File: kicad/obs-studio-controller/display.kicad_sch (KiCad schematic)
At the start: 3 parts, among them J4 Conn_Display, Q1 2N7002

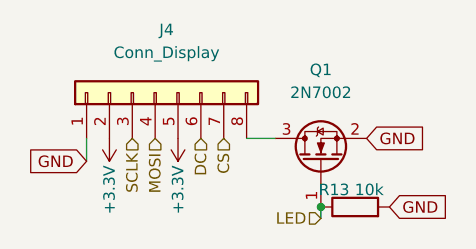
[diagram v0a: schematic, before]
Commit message: Routing complete
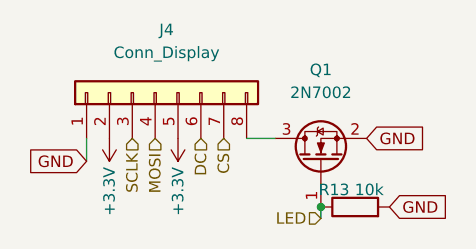
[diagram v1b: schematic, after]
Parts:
- J4: footprint Connector_PinHeader_2.54mm:PinHeader_1x08_P2.54mm_Vertical -> custom:DISPLAY
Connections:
- net +3.3V renamed +3V3
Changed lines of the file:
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@@
     (effects (font (size 1.27 1.27)) (justify right))
+  )
+  (symbol (lib_id "power:+3.3V") (at 34.925 30.48 180) (unit 1)
+    (in_bom yes) (on_board yes)
+    (property "Reference" "#PWR?" (id 0) (at 34.925 26.67 0)
+      (effects (font (size 1.27 1.27)) hide)
+    )
+    (property "Value" "+3.3V" (id 1) (at 34.925 33.655 90)
+      (effects (font (size 1.27 1.27)) (justify left))
+    )
+    (property "Footprint" "" (id 2) (at 34.925 30.48 0)
+      (effects (font (size 1.27 1.27)) hide)
+    )
+    (property "Datasheet" "" (id 3) (at 34.925 30.48 0)
+      (effects (font (size 1.27 1.27)) hide)
+    )
+    (pin "1")
   )
   (symbol (lib_id "Device:R") (at 54.61 38.1 90) (unit 1)
@@
     (pin "2")
   )
-  (symbol (lib_id "power:+3.3V") (at 34.925 30.48 180) (unit 1)
+  (symbol (lib_id "power:+3.3V") (at 27.305 30.48 180) (unit 1)
     (in_bom yes) (on_board yes)
-    (property "Reference" "#PWR0116" (id 0) (at 34.925 26.67 0)
+    (property "Reference" "#PWR?" (id 0) (at 27.305 26.67 0)
       (effects (font (size 1.27 1.27)) hide)
     )
-    (property "Value" "+3.3V" (id 1) (at 34.925 36.195 90))
-    (property "Footprint" "" (id 2) (at 34.925 30.48 0)
+    (property "Value" "+3.3V" (id 1) (at 27.305 33.655 90)
+      (effects (font (size 1.27 1.27)) (justify left))
+    )
+    (property "Footprint" "" (id 2) (at 27.305 30.48 0)
       (effects (font (size 1.27 1.27)) hide)
     )
-    (property "Datasheet" "" (id 3) (at 34.925 30.48 0)
+    (property "Datasheet" "" (id 3) (at 27.305 30.48 0)
       (effects (font (size 1.27 1.27)) hide)
     )
@@
     (property "Reference" "J4" (id 0) (at 33.655 18.415 90))
     (property "Value" "Conn_Display" (id 1) (at 33.655 20.955 90))
-    (property "Footprint" "Connector_PinHeader_2.54mm:PinHeader_1x08_P2.54mm_Vertical" (id 2) (at 32.385 25.4 0)
+    (property "Footprint" "custom:DISPLAY" (id 2) (at 32.385 25.4 0)
       (effects (font (size 1.27 1.27)) hide)
     )
@@
     (pin "8")
   )
-  (symbol (lib_id "power:+3.3V") (at 27.305 30.48 180) (unit 1)
-    (in_bom yes) (on_board yes)
-    (property "Reference" "#PWR0117" (id 0) (at 27.305 26.67 0)
-      (effects (font (size 1.27 1.27)) hide)
-    )
-    (property "Value" "+3.3V" (id 1) (at 27.305 36.195 90))
-    (property "Footprint" "" (id 2) (at 27.305 30.48 0)
-      (effects (font (size 1.27 1.27)) hide)
-    )
-    (property "Datasheet" "" (id 3) (at 27.305 30.48 0)
-      (effects (font (size 1.27 1.27)) hide)
-    )
-    (pin "1")
-  )
   (symbol (lib_id "Transistor_FET:2N7002") (at 50.8 33.02 90) (unit 1)
